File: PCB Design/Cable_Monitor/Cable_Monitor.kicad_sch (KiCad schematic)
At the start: 45 parts, among them J1 USB_B_Micro, P1 ${SIM.PARAMS}, P2 ${SIM.PARAMS}, Q1 BSS316N, SW1 ${SIM.PARAMS}, U1 SiP32508, U2 LD1117S33TR, U3 DRV5053_THT, U4 DRV5053_THT

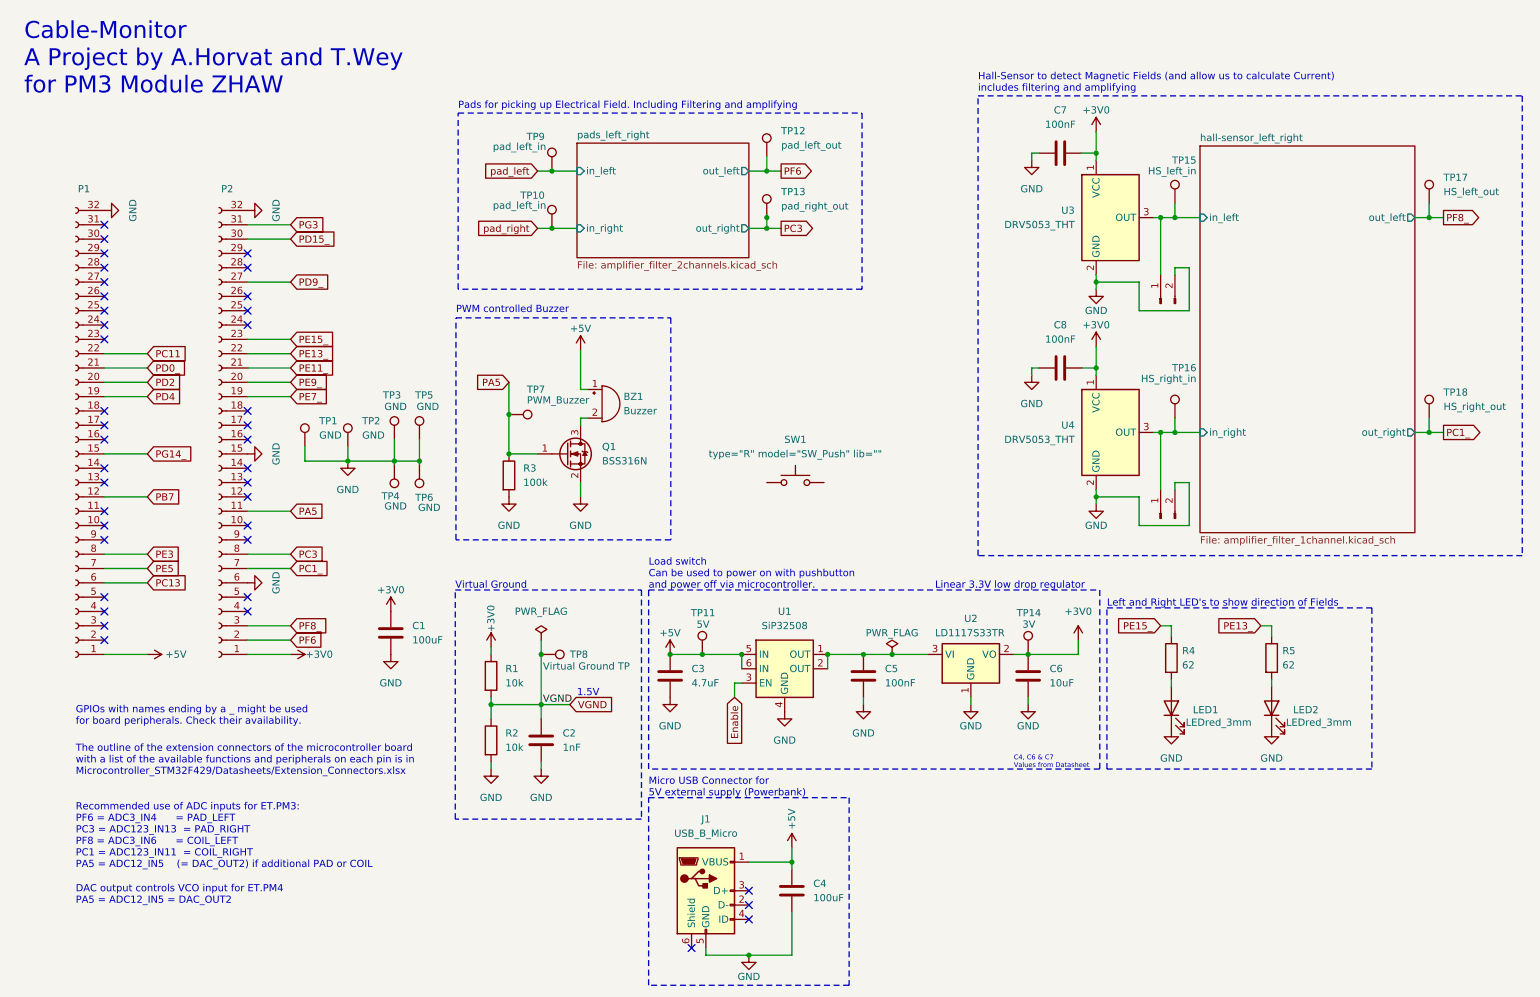
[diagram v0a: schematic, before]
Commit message: Update
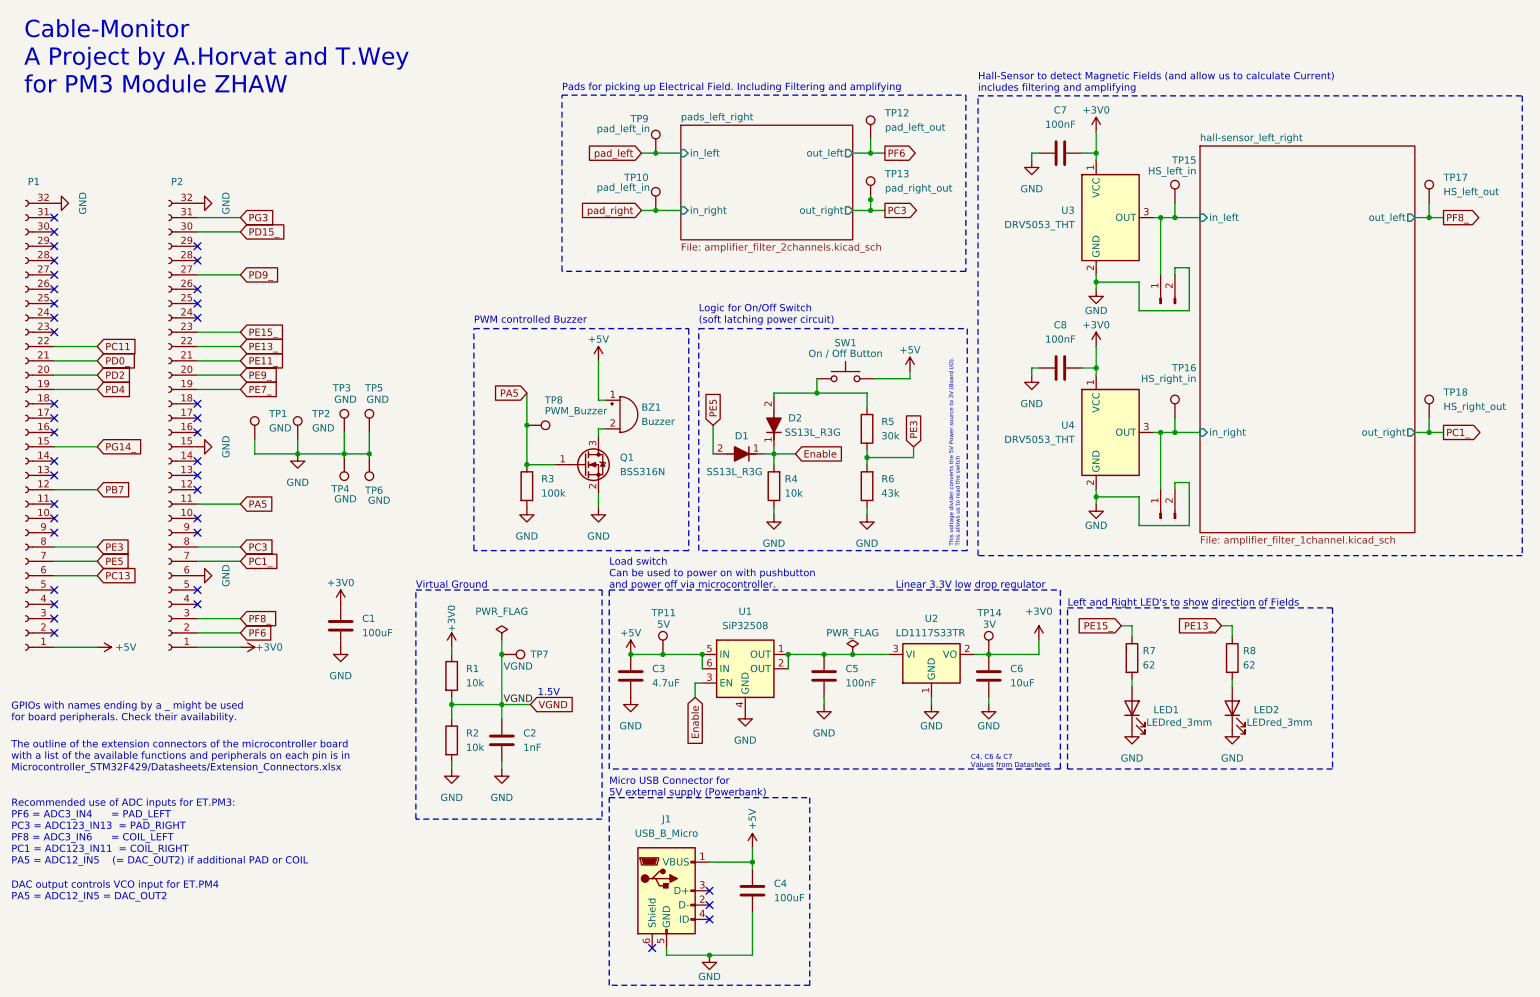
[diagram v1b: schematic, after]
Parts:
- added D1, D2: SS13L_R3G, SODFL3618X143N, symbol SS13L_R3G:SS13L_R3G
- added R4: 10k, Resistor_SMD:R_0805_2012Metric_Pad1.20x1.40mm_HandSolder, symbol Device:R
- added R5: 30k, Resistor_SMD:R_0805_2012Metric_Pad1.20x1.40mm_HandSolder, symbol Device:R
- added R6: 43k, Resistor_SMD:R_0805_2012Metric_Pad1.20x1.40mm_HandSolder, symbol Device:R
- SW1: value ${SIM.PARAMS} -> On / Off Button
- TP7: renamed from TP8; value Virtual Ground TP -> VGND
- renumbered Lconn1 to HS_Left1, Lconn2 to HS_right1, R4 to R7, R5 to R8, TP7 to TP8
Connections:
- net +5V: now also SW1.2
- net Enable: now also D1.1 (K), D2.1 (K), R4.2
- net GND: now also R4.1, R6.1
- net PE3: now also R5.2, R6.2
- net PE5: now also D1.2 (A)
- net at SW1.1: now also D2.2 (A), R5.1
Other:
- note added: "Logic for On/Off Switch (soft latching power circuit)"
- note added: "This voltage divider converts the 5V Power source to 3V (Board I/O). This allows us to read the switch"
- moved on the sheet: BZ1, C1, C2, C3, C4, C5, C6, J1, LED1, LED2, P1, P2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
